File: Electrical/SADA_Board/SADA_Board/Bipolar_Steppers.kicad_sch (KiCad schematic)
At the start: 55 parts, among them J10 171973-0004, J9 171973-0004, U6 STSPIN220, U7 STSPIN220

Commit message: ESD changes
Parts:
- D14, D15, D16, D17, D18, D19, D20, D21, D22, D23, D24, D25, D26, D27: footprint (none) -> Diode_SMD:D_0402_1005Metric
- TP13, TP14, TP15, TP16, TP17, TP18, TP19, TP20, TP21: footprint TestPoint:TestPoint_Pad_D1.5mm -> TestPoint:TestPoint_Pad_D1.0mm
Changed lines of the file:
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@@
       (effects (font (size 1.27 1.27)) (justify right) hide)
     )
-    (property "Footprint" "TestPoint:TestPoint_Pad_D1.5mm" (id 2) (at 188.976 68.58 0)
+    (property "Footprint" "TestPoint:TestPoint_Pad_D1.0mm" (id 2) (at 188.976 68.58 0)
       (effects (font (size 1.27 1.27)) hide)
     )
@@
       (effects (font (size 1.27 1.27)) hide)
     )
-    (property "Footprint" "" (id 2) (at 161.417 70.358 0)
+    (property "Footprint" "Diode_SMD:D_0402_1005Metric" (id 2) (at 161.417 70.358 0)
       (effects (font (size 1.27 1.27)) hide)
     )
@@
       (effects (font (size 1.27 1.27)) hide)
     )
-    (property "Footprint" "" (id 2) (at 163.068 109.855 0)
+    (property "Footprint" "Diode_SMD:D_0402_1005Metric" (id 2) (at 163.068 109.855 0)
       (effects (font (size 1.27 1.27)) hide)
     )
@@
       (effects (font (size 1.27 1.27)) hide)
     )
-    (property "Footprint" "" (id 2) (at 208.026 33.655 0)
+    (property "Footprint" "Diode_SMD:D_0402_1005Metric" (id 2) (at 208.026 33.655 0)
       (effects (font (size 1.27 1.27)) hide)
     )
@@
       (effects (font (size 1.27 1.27)) (justify right) hide)
     )
-    (property "Footprint" "TestPoint:TestPoint_Pad_D1.5mm" (id 2) (at 173.99 48.26 0)
+    (property "Footprint" "TestPoint:TestPoint_Pad_D1.0mm" (id 2) (at 173.99 48.26 0)
       (effects (font (size 1.27 1.27)) hide)
     )
@@
       (effects (font (size 1.27 1.27)) hide)
     )
-    (property "Footprint" "" (id 2) (at 163.703 147.32 0)
+    (property "Footprint" "Diode_SMD:D_0402_1005Metric" (id 2) (at 163.703 147.32 0)
       (effects (font (size 1.27 1.27)) hide)
     )
@@
       (effects (font (size 1.27 1.27)) hide)
     )
-    (property "Footprint" "" (id 2) (at 208.153 110.617 0)
+    (property "Footprint" "Diode_SMD:D_0402_1005Metric" (id 2) (at 208.153 110.617 0)
       (effects (font (size 1.27 1.27)) hide)
     )
@@
       (effects (font (size 1.27 1.27)) hide)
     )
-    (property "Footprint" "" (id 2) (at 179.451 77.978 0)
+    (property "Footprint" "Diode_SMD:D_0402_1005Metric" (id 2) (at 179.451 77.978 0)
       (effects (font (size 1.27 1.27)) hide)
     )
@@
       (effects (font (size 1.27 1.27)) hide)
     )
-    (property "Footprint" "" (id 2) (at 183.261 77.978 0)
+    (property "Footprint" "Diode_SMD:D_0402_1005Metric" (id 2) (at 183.261 77.978 0)
       (effects (font (size 1.27 1.27)) hide)
     )
@@
       (effects (font (size 1.27 1.27)) hide)
     )
-    (property "Footprint" "" (id 2) (at 167.513 147.32 0)
+    (property "Footprint" "Diode_SMD:D_0402_1005Metric" (id 2) (at 167.513 147.32 0)
       (effects (font (size 1.27 1.27)) hide)
     )
@@
       (effects (font (size 1.27 1.27)) hide)
     )
-    (property "Footprint" "" (id 2) (at 159.766 36.703 0)
+    (property "Footprint" "Diode_SMD:D_0402_1005Metric" (id 2) (at 159.766 36.703 0)
       (effects (font (size 1.27 1.27)) hide)
     )
@@
       (effects (font (size 1.27 1.27)) hide)
     )
-    (property "Footprint" "" (id 2) (at 163.068 113.665 0)
+    (property "Footprint" "Diode_SMD:D_0402_1005Metric" (id 2) (at 163.068 113.665 0)
       (effects (font (size 1.27 1.27)) hide)
     )
@@
       (effects (font (size 1.27 1.27)) (justify right) hide)
     )
-    (property "Footprint" "TestPoint:TestPoint_Pad_D1.5mm" (id 2) (at 229.362 63.5 0)
+    (property "Footprint" "TestPoint:TestPoint_Pad_D1.0mm" (id 2) (at 229.362 63.5 0)
       (effects (font (size 1.27 1.27)) hide)
     )
@@
       (effects (font (size 1.27 1.27)) hide)
     )
-    (property "Footprint" "" (id 2) (at 180.975 154.94 0)
+    (property "Footprint" "Diode_SMD:D_0402_1005Metric" (id 2) (at 180.975 154.94 0)
       (effects (font (size 1.27 1.27)) hide)
     )
@@
       (effects (font (size 1.27 1.27)) hide)
     )
-    (property "Footprint" "" (id 2) (at 174.879 154.94 0)
+    (property "Footprint" "Diode_SMD:D_0402_1005Metric" (id 2) (at 174.879 154.94 0)
       (effects (font (size 1.27 1.27)) hide)
     )
@@
       (effects (font (size 1.27 1.27)) (justify right) hide)
     )
-    (property "Footprint" "TestPoint:TestPoint_Pad_D1.5mm" (id 2) (at 229.362 68.58 0)
+    (property "Footprint" "TestPoint:TestPoint_Pad_D1.0mm" (id 2) (at 229.362 68.58 0)
       (effects (font (size 1.27 1.27)) hide)
     )
@@
       (effects (font (size 1.27 1.27)) (justify right) hide)
     )
-    (property "Footprint" "TestPoint:TestPoint_Pad_D1.5mm" (id 2) (at 229.362 66.04 0)
+    (property "Footprint" "TestPoint:TestPoint_Pad_D1.0mm" (id 2) (at 229.362 66.04 0)
       (effects (font (size 1.27 1.27)) hide)
     )
@@
       (effects (font (size 1.27 1.27)) hide)
     )
-    (property "Footprint" "" (id 2) (at 159.766 32.893 0)
+    (property "Footprint" "Diode_SMD:D_0402_1005Metric" (id 2) (at 159.766 32.893 0)
       (effects (font (size 1.27 1.27)) hide)
     )
@@
       (effects (font (size 1.27 1.27)) (justify right) hide)
     )
-    (property "Footprint" "TestPoint:TestPoint_Pad_D1.5mm" (id 2) (at 229.87 53.34 0)
+    (property "Footprint" "TestPoint:TestPoint_Pad_D1.0mm" (id 2) (at 229.87 53.34 0)
       (effects (font (size 1.27 1.27)) hide)
     )
@@
       (effects (font (size 1.27 1.27)) (justify right) hide)
     )
-    (property "Footprint" "TestPoint:TestPoint_Pad_D1.5mm" (id 2) (at 184.15 45.72 0)
+    (property "Footprint" "TestPoint:TestPoint_Pad_D1.0mm" (id 2) (at 184.15 45.72 0)
       (effects (font (size 1.27 1.27)) hide)
     )
@@
       (effects (font (size 1.27 1.27)) (justify right) hide)
     )
-    (property "Footprint" "TestPoint:TestPoint_Pad_D1.5mm" (id 2) (at 229.87 50.8 0)
+    (property "Footprint" "TestPoint:TestPoint_Pad_D1.0mm" (id 2) (at 229.87 50.8 0)
       (effects (font (size 1.27 1.27)) hide)
     )
@@
       (effects (font (size 1.27 1.27)) hide)
     )
-    (property "Footprint" "" (id 2) (at 157.607 70.358 0)
+    (property "Footprint" "Diode_SMD:D_0402_1005Metric" (id 2) (at 157.607 70.358 0)
       (effects (font (size 1.27 1.27)) hide)
     )
@@
       (effects (font (size 1.27 1.27)) (justify right) hide)
     )
-    (property "Footprint" "TestPoint:TestPoint_Pad_D1.5mm" (id 2) (at 229.87 55.88 0)
-      (effects (font (size 1.27 1.27)) hide)
-    )
+    (property "Footprint" "TestPoint:TestPoint_Pad_D1.0mm" (id 2) (at 229.87 55.88 0)
+      (effects (font (size 1.27 1.27)) hide)
+    )

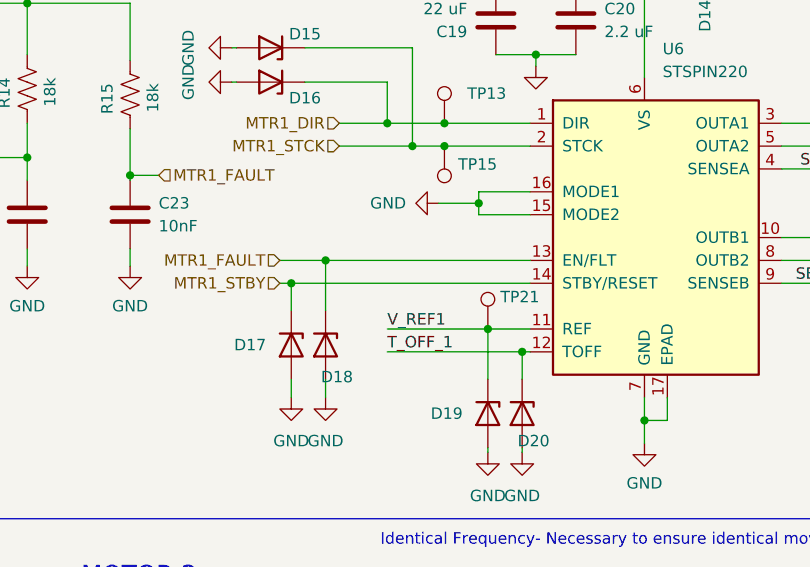
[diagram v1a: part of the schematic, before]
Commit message: layout prog
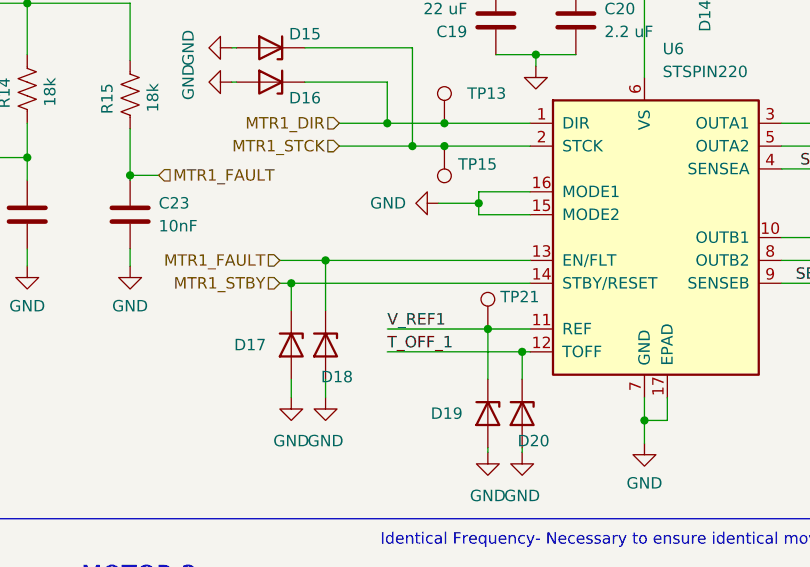
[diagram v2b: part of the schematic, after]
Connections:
- net MTR1_FAULT: now also D18.1 (K)
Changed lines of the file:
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@@
   (junction (at 201.295 155.702) (diameter 0) (color 0 0 0 0)
   )
+  (junction (at 165.862 60.96) (diameter 0) (color 0 0 0 0)
+  )
   (junction (at 201.295 106.172) (diameter 0) (color 0 0 0 0)
   )
@@
   (junction (at 183.896 68.58) (diameter 0) (color 0 0 0 0)
   )
-  (junction (at 165.8671 60.9599) (diameter 0) (color 0 0 0 0)
-  )
   (junction (at 144.145 126.365) (diameter 0) (color 0 0 0 0)
   )
@@
     (stroke (width 0) (type default) (color 0 0 0 0))
   )
-  (wire (pts (xy 165.8671 60.9599) (xy 165.862 66.548))
-    (stroke (width 0) (type default) (color 0 0 0 0))
-  )
   (wire (pts (xy 34.925 31.75) (xy 34.925 38.1))
     (stroke (width 0) (type default) (color 0 0 0 0))
@@
     (stroke (width 0) (type default) (color 0 0 0 0))
   )
-  (wire (pts (xy 160.782 60.96) (xy 188.595 60.96))
+  (wire (pts (xy 160.782 60.96) (xy 165.862 60.96))
     (stroke (width 0) (type default) (color 0 0 0 0))
   )
@@
     (stroke (width 0) (type default) (color 0 0 0 0))
   )
+  (wire (pts (xy 165.862 60.96) (xy 165.862 66.548))
+    (stroke (width 0) (type default) (color 0 0 0 0))
+  )
   (wire (pts (xy 129.54 126.365) (xy 132.715 126.365))
     (stroke (width 0) (type default) (color 0 0 0 0))
@@
     (stroke (width 0) (type default) (color 0 0 0 0))
   )
+  (wire (pts (xy 165.862 60.96) (xy 188.595 60.96))
+    (stroke (width 0) (type default) (color 0 0 0 0))
+  )
